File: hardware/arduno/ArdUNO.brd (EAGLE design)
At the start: 33.3 x 30.2 mm, 20 parts, among them IC1 MEGA644P, Q1 8,0 MHz

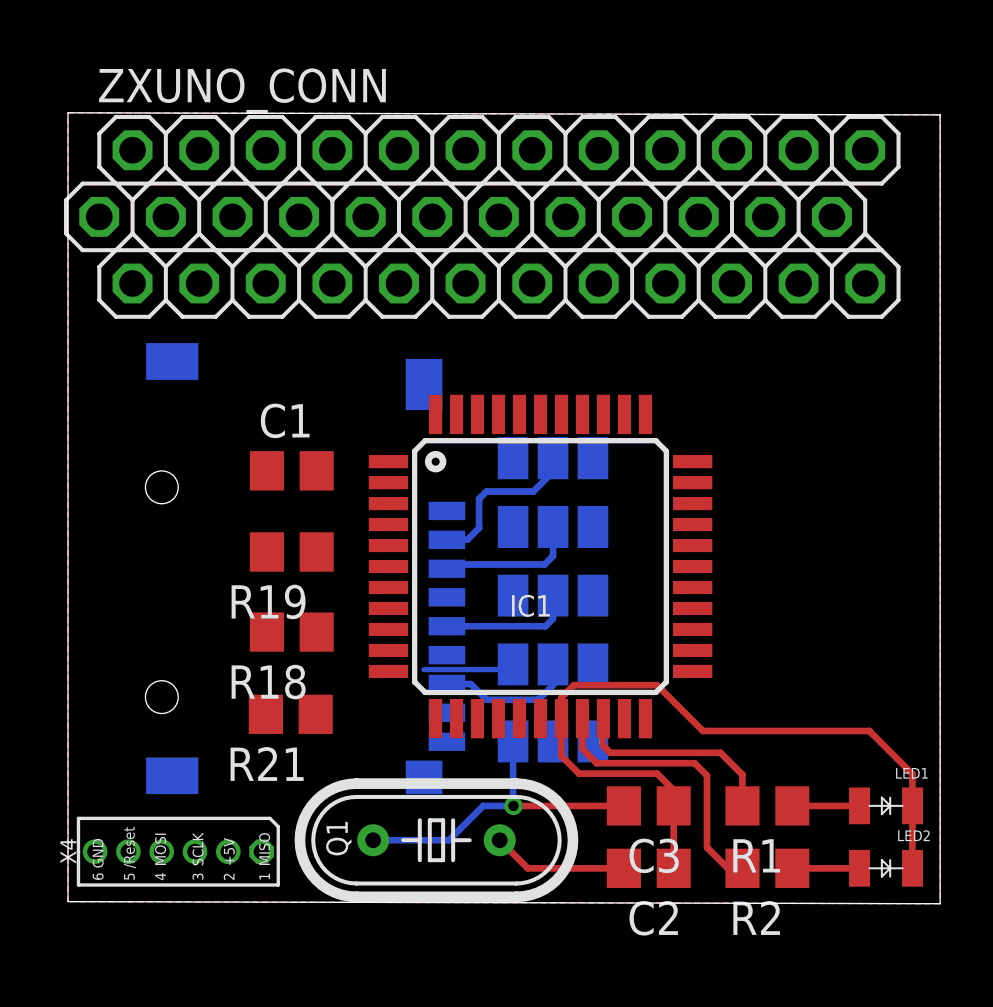
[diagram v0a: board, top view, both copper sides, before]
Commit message: Finalizo diseño
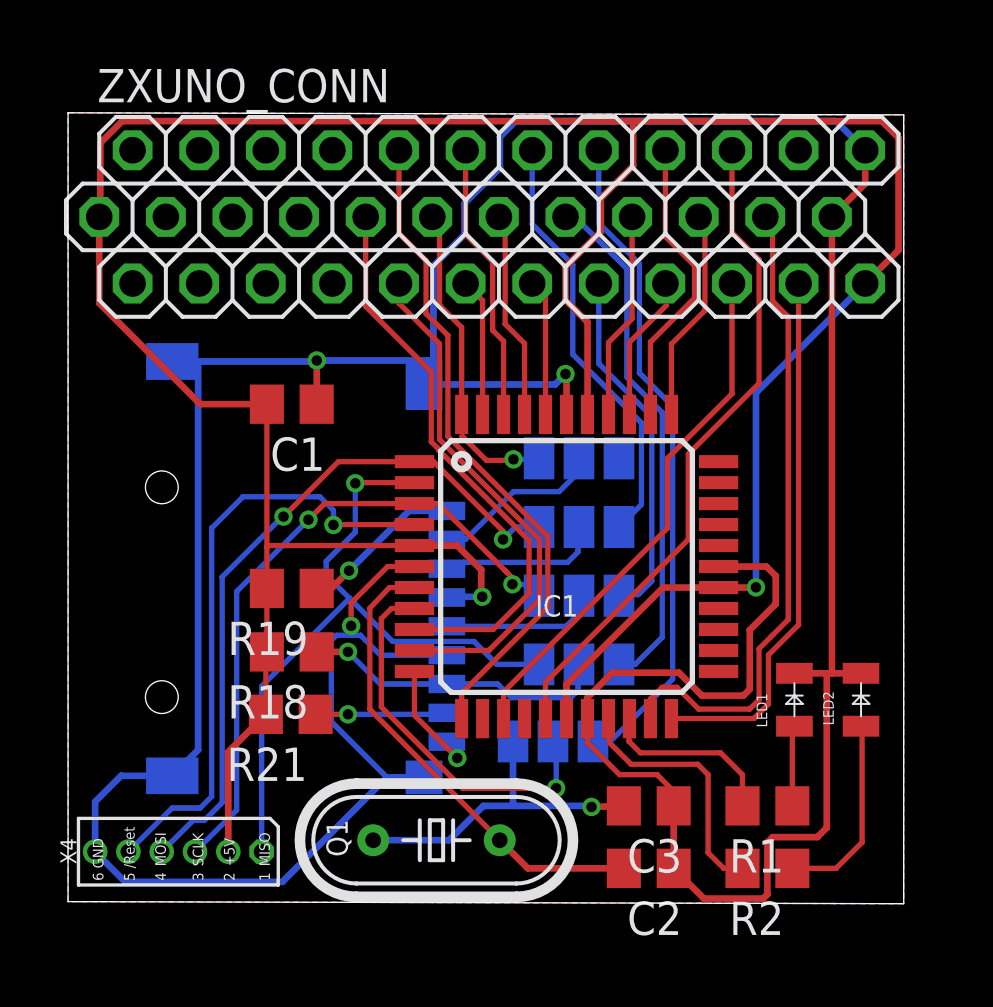
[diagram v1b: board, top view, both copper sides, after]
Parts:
- moved LED2 6.50 mm to (30.2, 7.70), turned to 270 degrees
- moved LED1 5.35 mm to (27.7, 7.70), turned to 270 degrees
- moved C1 2.54 mm to (8.53, 19.0), turned to 180 degrees
- moved R19 1.39 mm to (8.53, 11.9)
- moved IC1 0.99 mm to (19.0, 12.8)
- moved SJ2 0.99 mm to (19.5, 16.9)
- moved SJ3 0.99 mm to (19.5, 14.3)
- moved SJ4 0.99 mm to (19.5, 11.7)
- moved SJ5 0.99 mm to (19.5, 9.05)
- moved R18 0.75 mm to (8.53, 9.53)
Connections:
- net N$15 renamed FSS
- removed net N$14: SJ4.3
- removed net N$16: SJ3.3
- removed net N$17: SJ1.1
- removed net P16: ZXUNO_CONN.P16
- removed net P17: ZXUNO_CONN.P17
- removed net P18: ZXUNO_CONN.P18
- new net FMISO: SJ5.3, ZXUNO_CONN.P26
- new net FMOSI: SJ3.3, ZXUNO_CONN.P24
- new net FSCK: SJ4.3, ZXUNO_CONN.P25
- new net OSC: SJ1.1, ZXUNO_CONN.P27
- new net P23: IC1.41, ZXUNO_CONN.P23
- net ATN: now also ZXUNO_CONN.P29
- net CLK: now also ZXUNO_CONN.P30
- net DATA: now also ZXUNO_CONN.P28
- net DISKSWITCH: now also ZXUNO_CONN.P34
- net IECRESERVE: now also ZXUNO_CONN.P32
- net IEC_10/11: now also ZXUNO_CONN.P31
- net IEC_8/9: now also ZXUNO_CONN.P33
- net P19: now also IC1.43
- net P20: now also IC1.44
- net P21: now also IC1.42
- net P22: now also IC1.40
- net RESERVE: now also ZXUNO_CONN.P35
- net RXD0: now also ZXUNO_CONN.P17
- net SS: no longer IC1.44
- net TXD0: now also ZXUNO_CONN.P16
- net TXD1: now also ZXUNO_CONN.P18
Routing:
- net GND: track 28.6 -> 156.0 mm, vias 0 -> 3
- net +3V3: track 0.00 -> 117.3 mm, vias 0 -> 2
- net MOSI: track 0.00 -> 27.3 mm, vias 0 -> 2
- net IEC_8/9: track 0.00 -> 25.5 mm
- net TXD1: track 0.00 -> 25.4 mm
- net OSC: track 0.00 -> 25.4 mm
- net SCK: track 0.00 -> 25.1 mm, vias 0 -> 2
- net RESERVE: track 0.00 -> 24.8 mm
- net MISO: track 3.48 -> 26.8 mm, vias 0 -> 1
- net /RESET: track 0.00 -> 23.3 mm, vias 0 -> 1
- net RXD0: track 0.00 -> 21.9 mm
- net DISKSWITCH: track 0.00 -> 20.4 mm
- net IEC_10/11: track 0.00 -> 20.2 mm
- net TXD0: track 0.00 -> 19.9 mm
- net FMISO: track 0.00 -> 19.9 mm
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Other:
- board size 33.3 x 30.2 mm -> 31.9 x 30.2 mm

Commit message: Actualizo varios
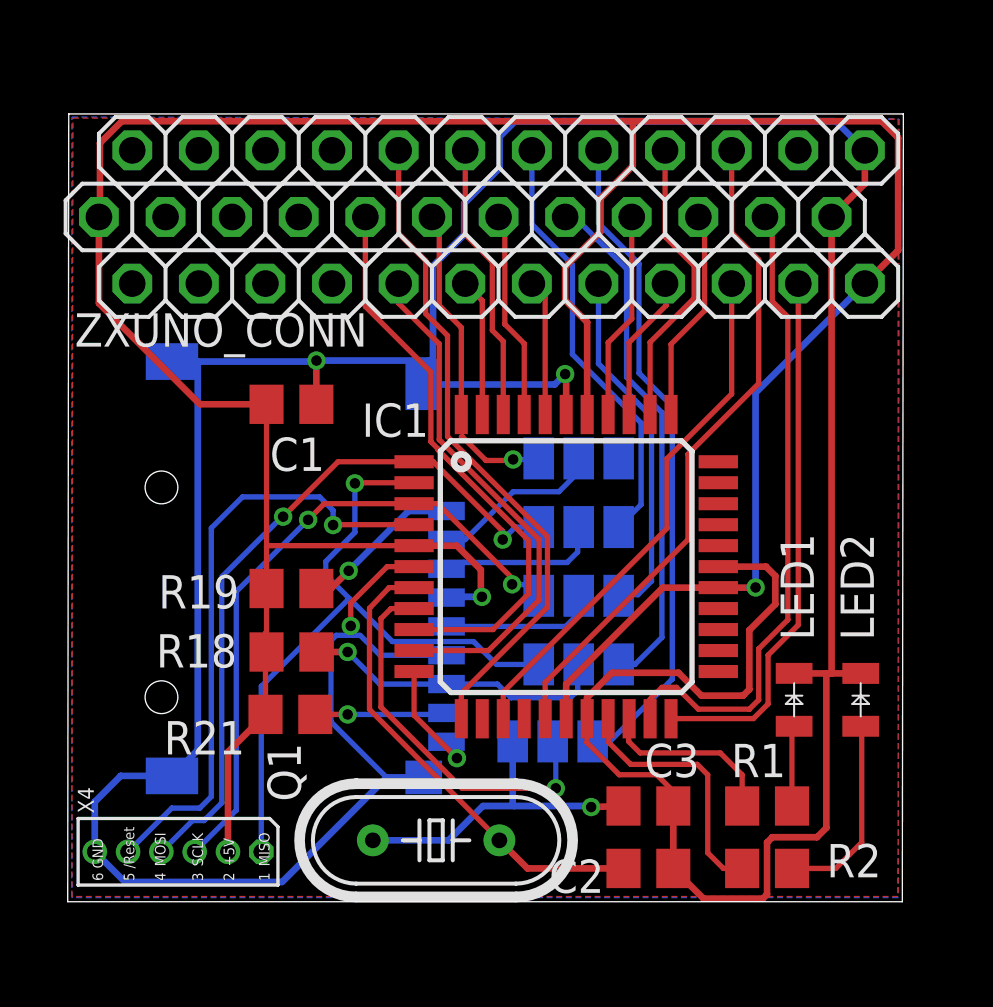
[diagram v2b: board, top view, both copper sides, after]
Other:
- board size 31.9 x 30.2 mm -> 31.9 x 30 mm
